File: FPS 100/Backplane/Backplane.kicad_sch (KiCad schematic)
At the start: 27 parts

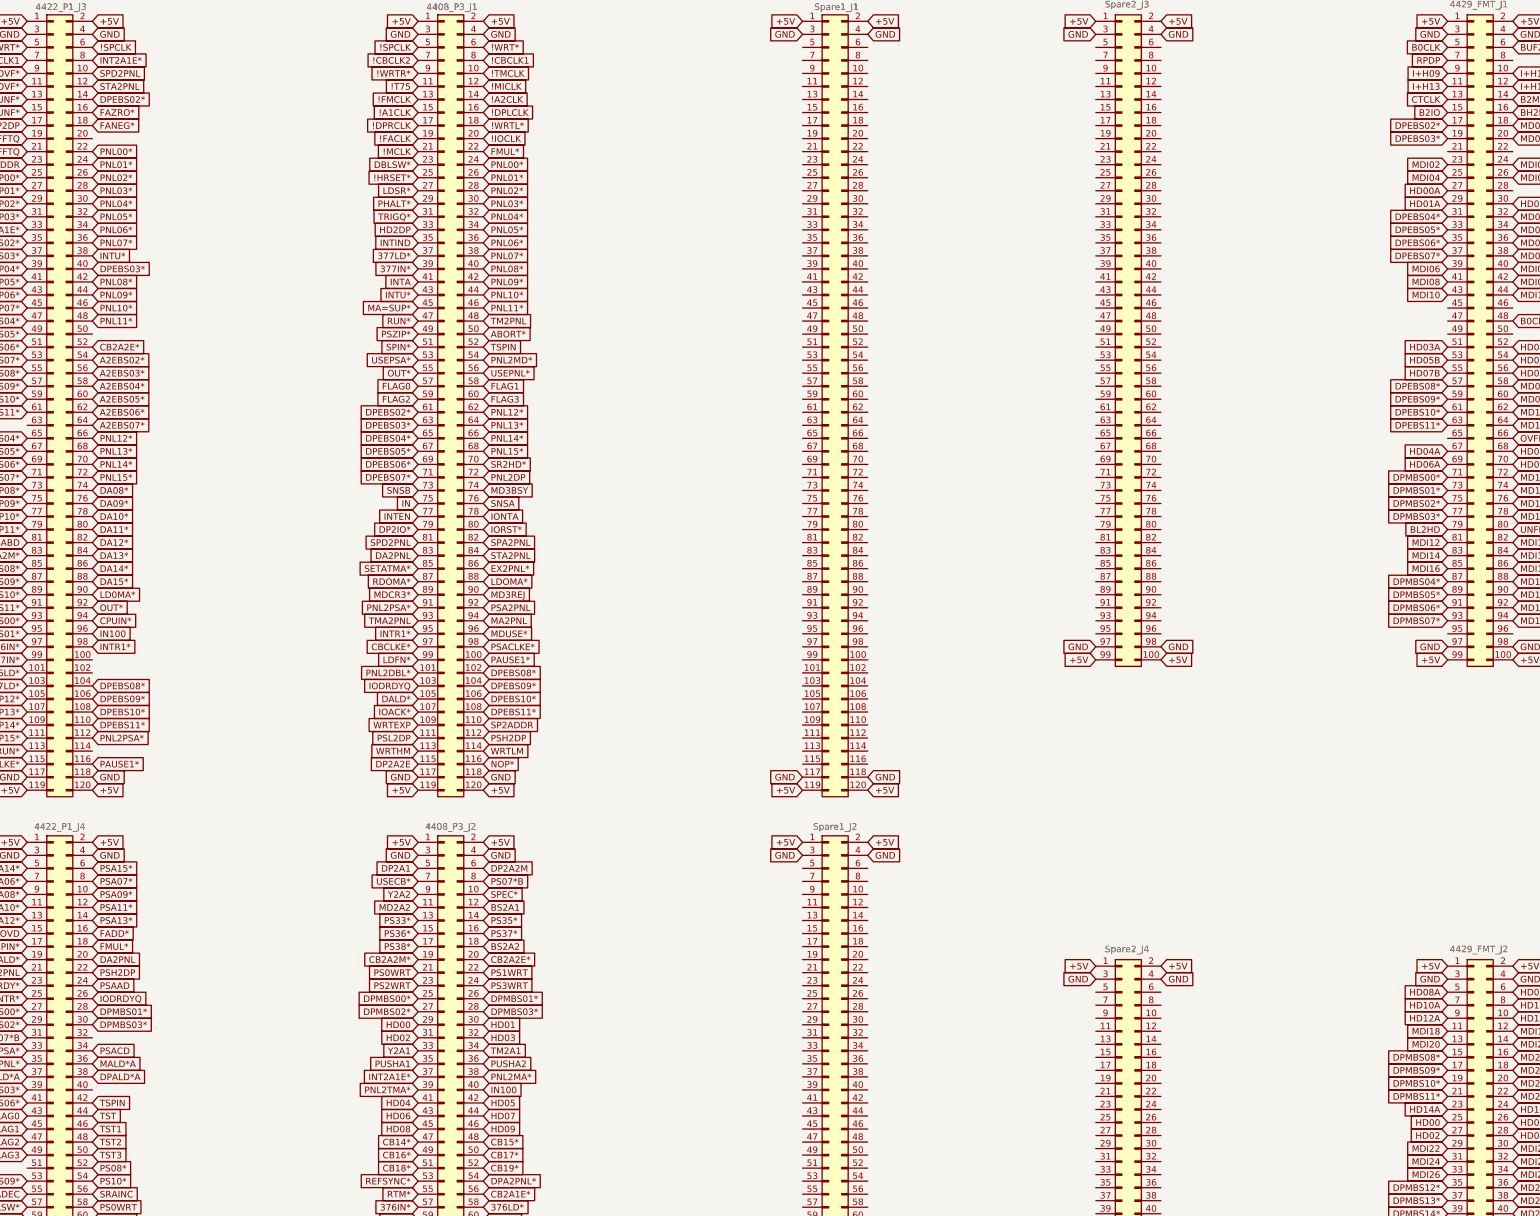
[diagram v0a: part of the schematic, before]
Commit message: 2026/1/10
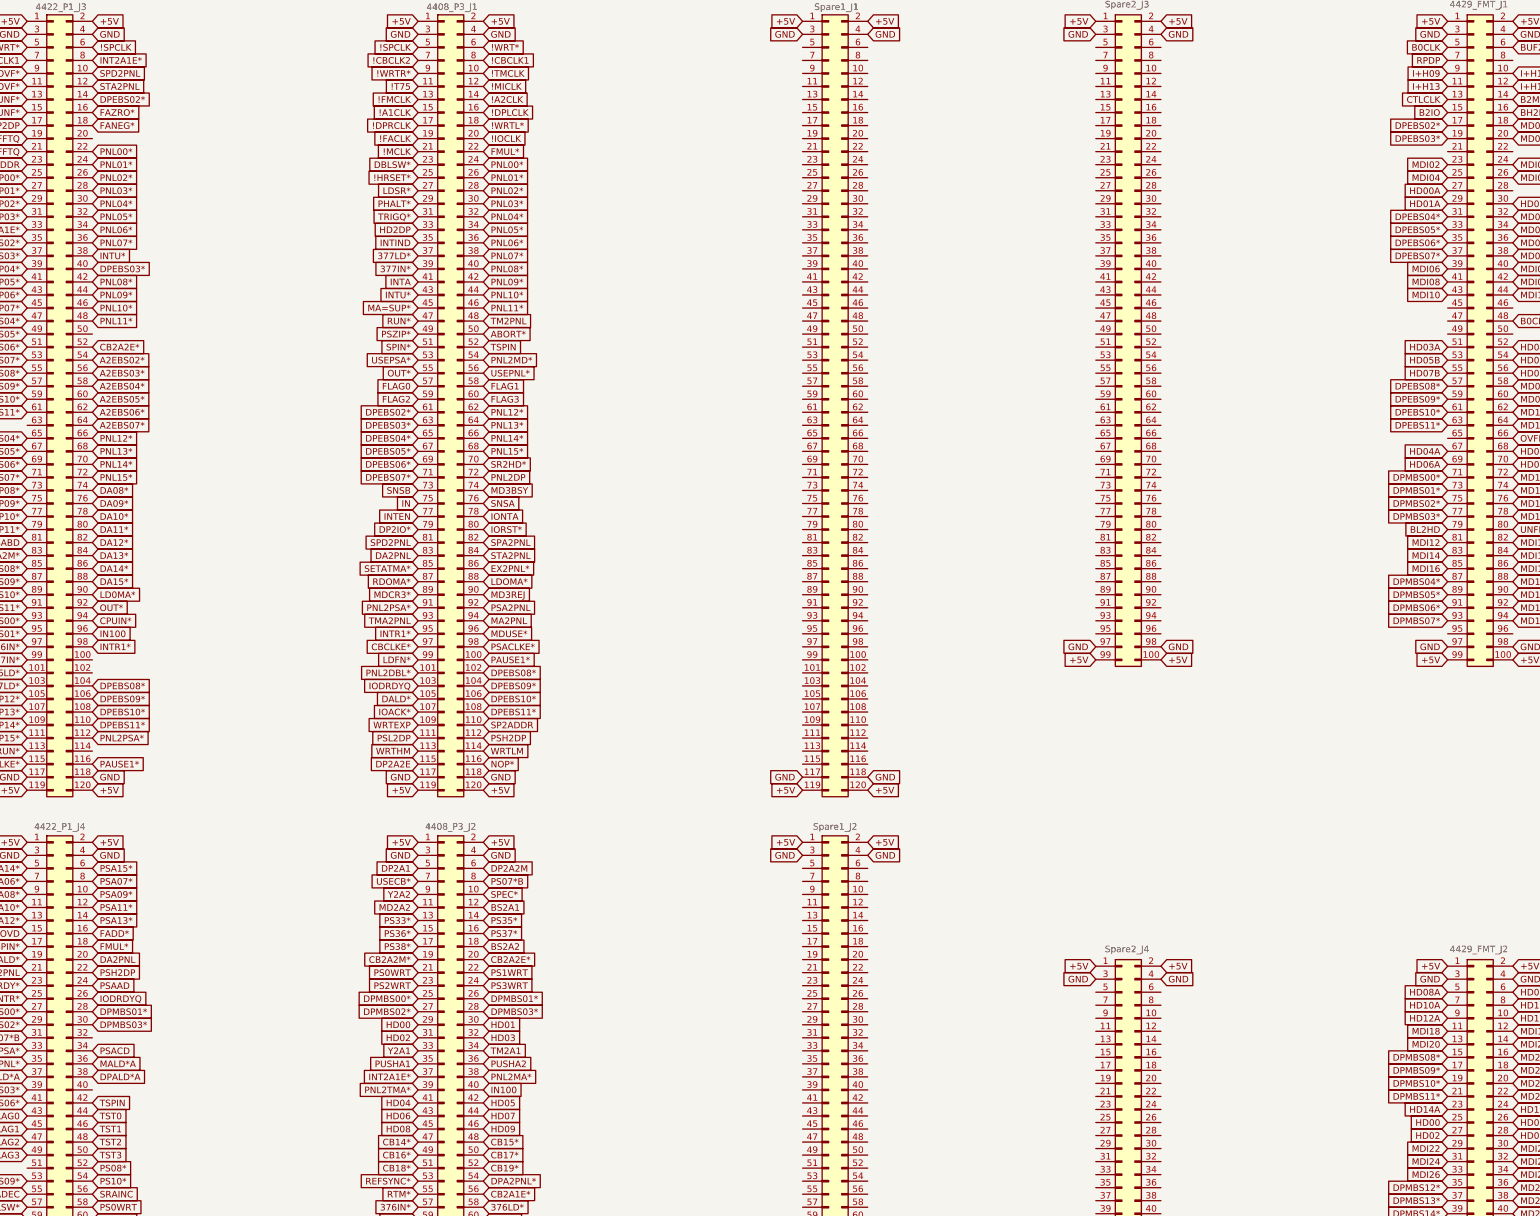
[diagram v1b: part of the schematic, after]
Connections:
- net CTCLK is gone; now on net CTLCLK: 4429_FMT_J1.13
- net TST renamed TST0
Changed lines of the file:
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@@
 		)
 	)
-	(global_label "CTCLK"
+	(global_label "CTLCLK"
 		(shape input)
 		(at 908.05 77.47 180)
@@
 		)
 		(property "Intersheetrefs" "${INTERSHEET_REFS}"
-			(at 899.2591 77.47 0)
+			(at 898.231 77.47 0)
 			(effects
 				(font
@@
 		)
 	)
-	(global_label "TST"
+	(global_label "TST0"
 		(shape input)
 		(at 643.89 275.59 0)
@@
 		)
 		(property "Intersheetrefs" "${INTERSHEET_REFS}"
-			(at 650.0199 275.59 0)
+			(at 651.2294 275.59 0)
 			(effects
 				(font

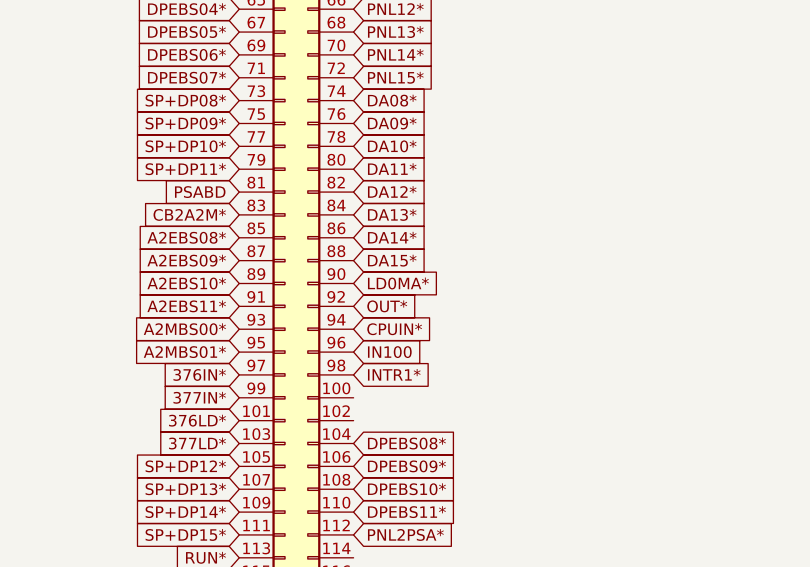
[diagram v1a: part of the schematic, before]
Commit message: 2026/1/15
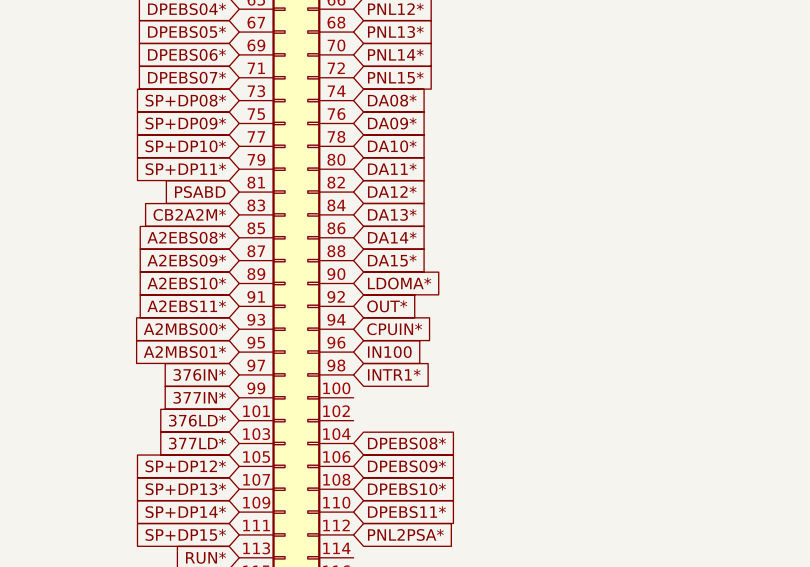
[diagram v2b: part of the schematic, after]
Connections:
- net LD0MA* is gone; now on net LDOMA*: 4422_P1_J3.90
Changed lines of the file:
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@@
 		)
 	)
-	(global_label "LD0MA*"
+	(global_label "LDOMA*"
 		(shape input)
 		(at 643.89 173.99 0)
@@
 		)
 		(property "Intersheetrefs" "${INTERSHEET_REFS}"
-			(at 653.8904 173.99 0)
+			(at 654.0114 173.99 0)
 			(effects
 				(font
